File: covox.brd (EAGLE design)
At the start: 80 x 50 mm, 26 parts, among them CN1 POWERJACK, IC1 74HCT373N, IC2 74HC164N

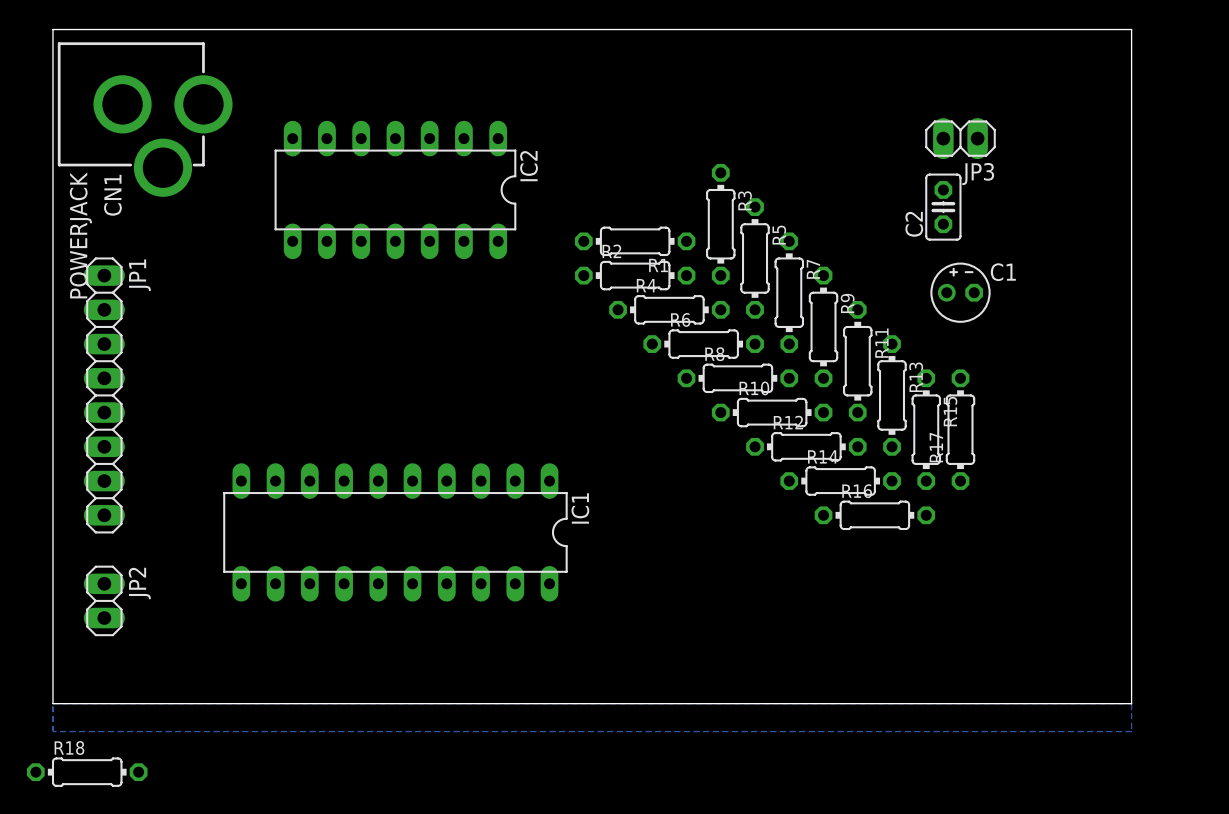
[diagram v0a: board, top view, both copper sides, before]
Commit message: Updates...
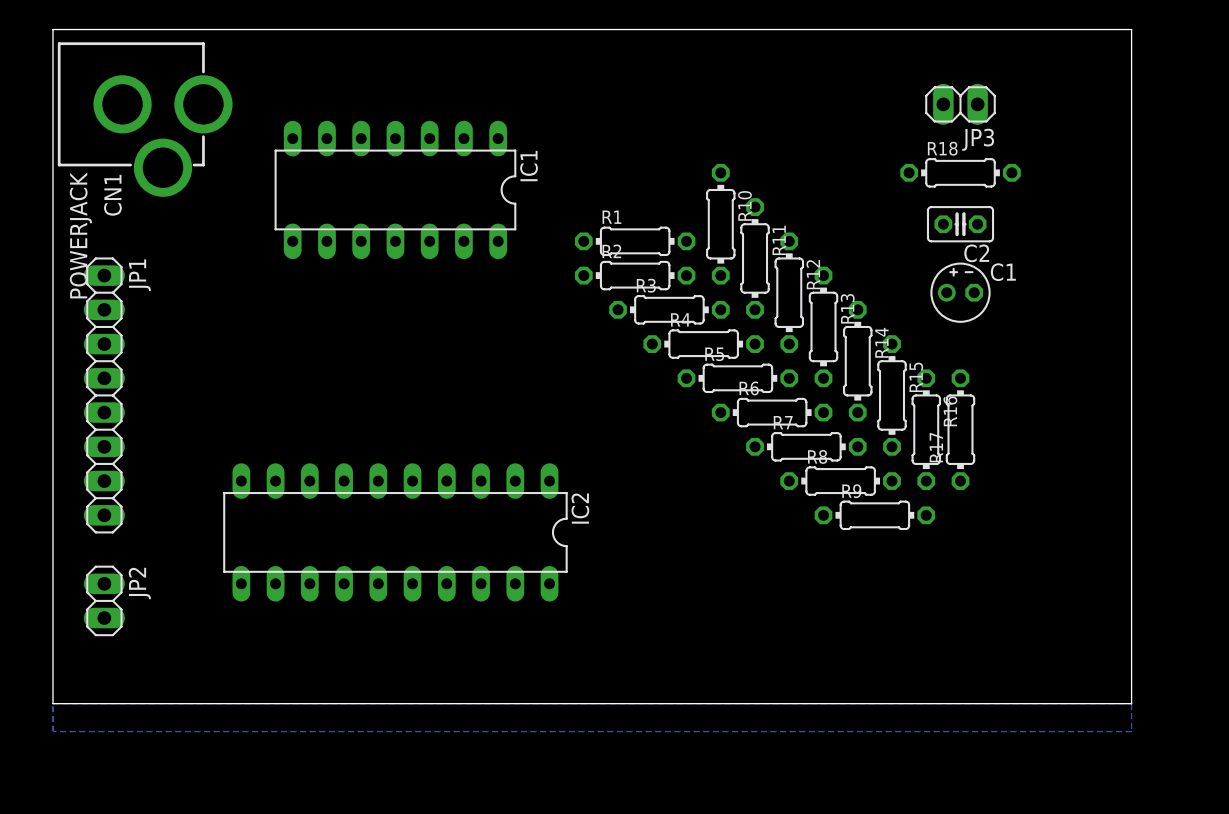
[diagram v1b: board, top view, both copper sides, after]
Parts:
- IC1: value 74HCT373N -> 74HC164N; device 74xx-eu:DIL20 -> 74xx-eu:DIL14
- IC2: value 74HC164N -> 74HCT373N; device 74xx-eu:DIL14 -> 74xx-eu:DIL20
- R10, R12, R14, R16: value 15k -> 7k5
- R3, R5, R7, R9: value 7k5 -> 15k
- moved R18 78.6 mm to (67.3, 39.4)
- moved IC1 25.4 mm to (25.4, 38.1)
- moved IC2 25.4 mm to (25.4, 12.7)
- moved R10 14.5 mm to (49.5, 35.6), turned to 270 degrees
- moved R9 14.5 mm to (61.0, 14.0), turned to 0 degrees
- moved R12 11.5 mm to (54.6, 30.5), turned to 270 degrees
- moved R7 11.5 mm to (55.9, 19.1), turned to 0 degrees
- moved R11 10.8 mm to (52.1, 33.0)
- moved R8 10.8 mm to (58.4, 16.5)
- moved R5 8.98 mm to (50.8, 24.1), turned to 0 degrees
- moved R14 8.98 mm to (59.7, 25.4), turned to 270 degrees
- moved R3 7.41 mm to (45.7, 29.2), turned to 0 degrees
- moved R16 7.41 mm to (64.8, 20.3), turned to 270 degrees
- moved R6 7.18 mm to (53.3, 21.6)
- moved R13 7.18 mm to (57.1, 27.9)
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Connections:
- net GND: now also IC1.7, IC2.10, R1.1; no longer IC1.10, IC2.7, R1.2
- net N$1: now also R1.2, R10.1; no longer R1.1, R3.1
- net N$10: now also IC2.6, R4.1; no longer IC1.6, R6.1
- net N$11: now also IC2.9, R5.1; no longer IC1.9, R8.1
- net N$12: now also IC2.12, R6.1; no longer IC1.12, R10.1
- net N$13: now also IC2.15, R7.1; no longer IC1.15, R12.1
- net N$14: now also IC2.16, R8.1; no longer IC1.16, R14.1
- net N$15: now also IC2.19, R9.1; no longer IC1.19, R16.1
- net N$17: now also R9.2; no longer R15.2
- net N$2: now also R10.2, R11.1; no longer R4.2, R5.1
- net N$20: now also IC1.5, IC2.7; no longer IC1.7, IC2.5
- net N$21: now also IC1.6, IC2.8; no longer IC1.8, IC2.6
- net N$22: now also IC1.10, IC2.13; no longer IC1.13, IC2.10
- net N$23: now also IC1.11, IC2.14; no longer IC1.14, IC2.11
- net N$24: now also IC1.12, IC2.17; no longer IC1.17, IC2.12
- net N$25: now also IC1.13, IC2.18; no longer IC1.18, IC2.13
- net N$26: now also IC2.1; no longer IC1.1
- net N$27: now also IC2.11; no longer IC1.11
- net N$3: now also R11.2, R12.1, R4.2; no longer R5.2, R6.2, R7.1
- net N$4: now also R12.2, R13.1, R5.2; no longer R7.2, R8.2, R9.1
- net N$5: now also R13.2, R14.1, R6.2; no longer R10.2, R11.1, R9.2
- net N$6: now also R14.2, R15.1, R7.2; no longer R11.2, R12.2, R13.1
- net N$7: now also R15.2, R16.1, R8.2; no longer R13.2, R14.2, R15.1
- net N$8: now also IC2.2; no longer IC1.2
- net N$9: now also IC2.5, R3.1; no longer IC1.5, R4.1
- net VCC: now also IC1.14, IC2.20; no longer IC1.20, IC2.14

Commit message: Updates...
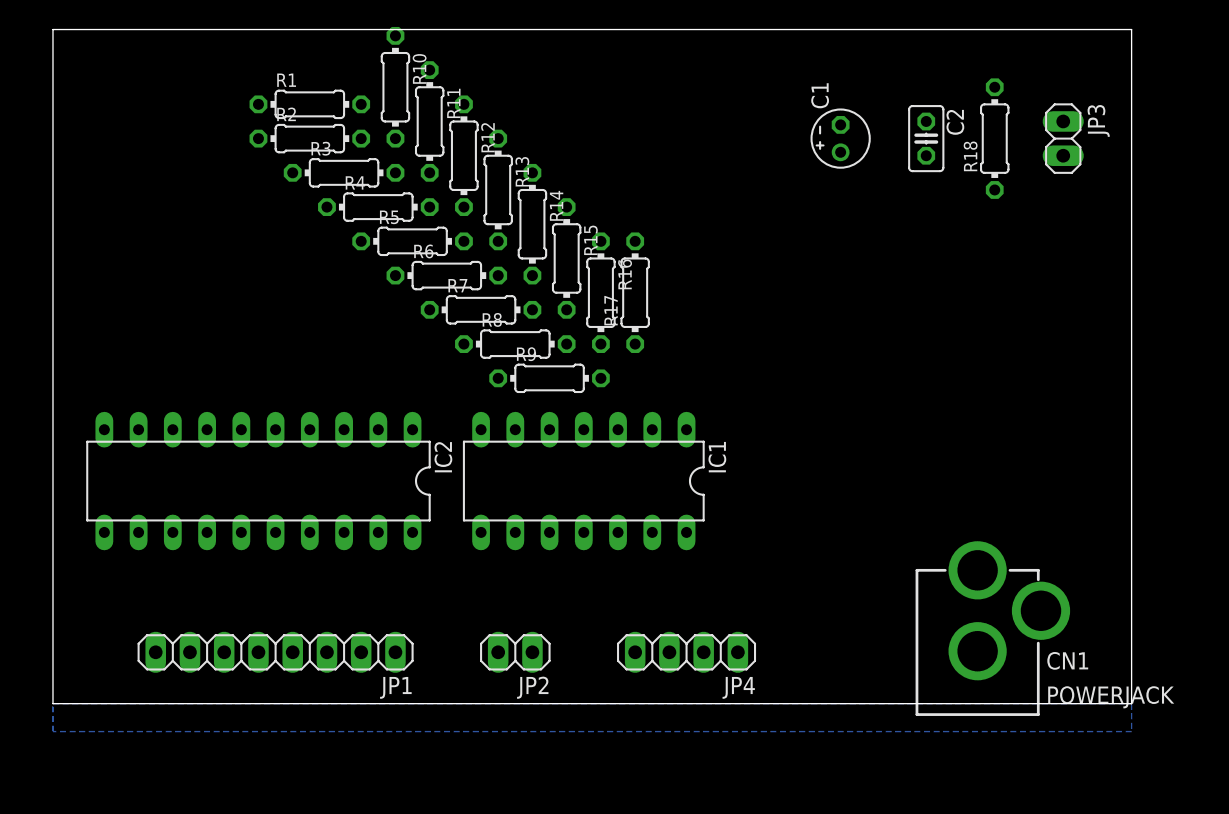
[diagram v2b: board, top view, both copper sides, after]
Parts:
- added JP4: SER-IN, pinhead:1X04
- JP1: value (none) -> PAR-IN
- JP2: value (none) -> LATCH
- moved CN1 85.9 mm to (68.6, -3.81), turned to 0 degrees
- moved JP2 30.7 mm to (34.3, 3.81), turned to 180 degrees
- moved R10 26.2 mm to (25.4, 45.7)
- moved R17 26.2 mm to (43.2, 30.5)
- moved R6 26.2 mm to (29.2, 31.8)
- moved R7 26.2 mm to (31.8, 29.2)
- moved R8 26.2 mm to (34.3, 26.7)
- moved R9 26.2 mm to (36.8, 24.1)
- moved R1 26.2 mm to (19.1, 44.5)
- moved R11 26.2 mm to (27.9, 43.2)
- moved R12 26.2 mm to (30.5, 40.6)
- moved R14 26.2 mm to (35.6, 35.6)
- moved R15 26.2 mm to (38.1, 33.0)
- moved R2 26.2 mm to (19.1, 41.9)
- moved R3 26.2 mm to (21.6, 39.4)
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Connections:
- new net N$16: IC1.1, JP4.1
- new net N$29: IC1.2, JP4.2
- new net N$30: IC1.9, JP4.4
- new net N$31: IC1.8, JP4.3
